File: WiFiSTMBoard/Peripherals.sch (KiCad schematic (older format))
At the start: 7 parts

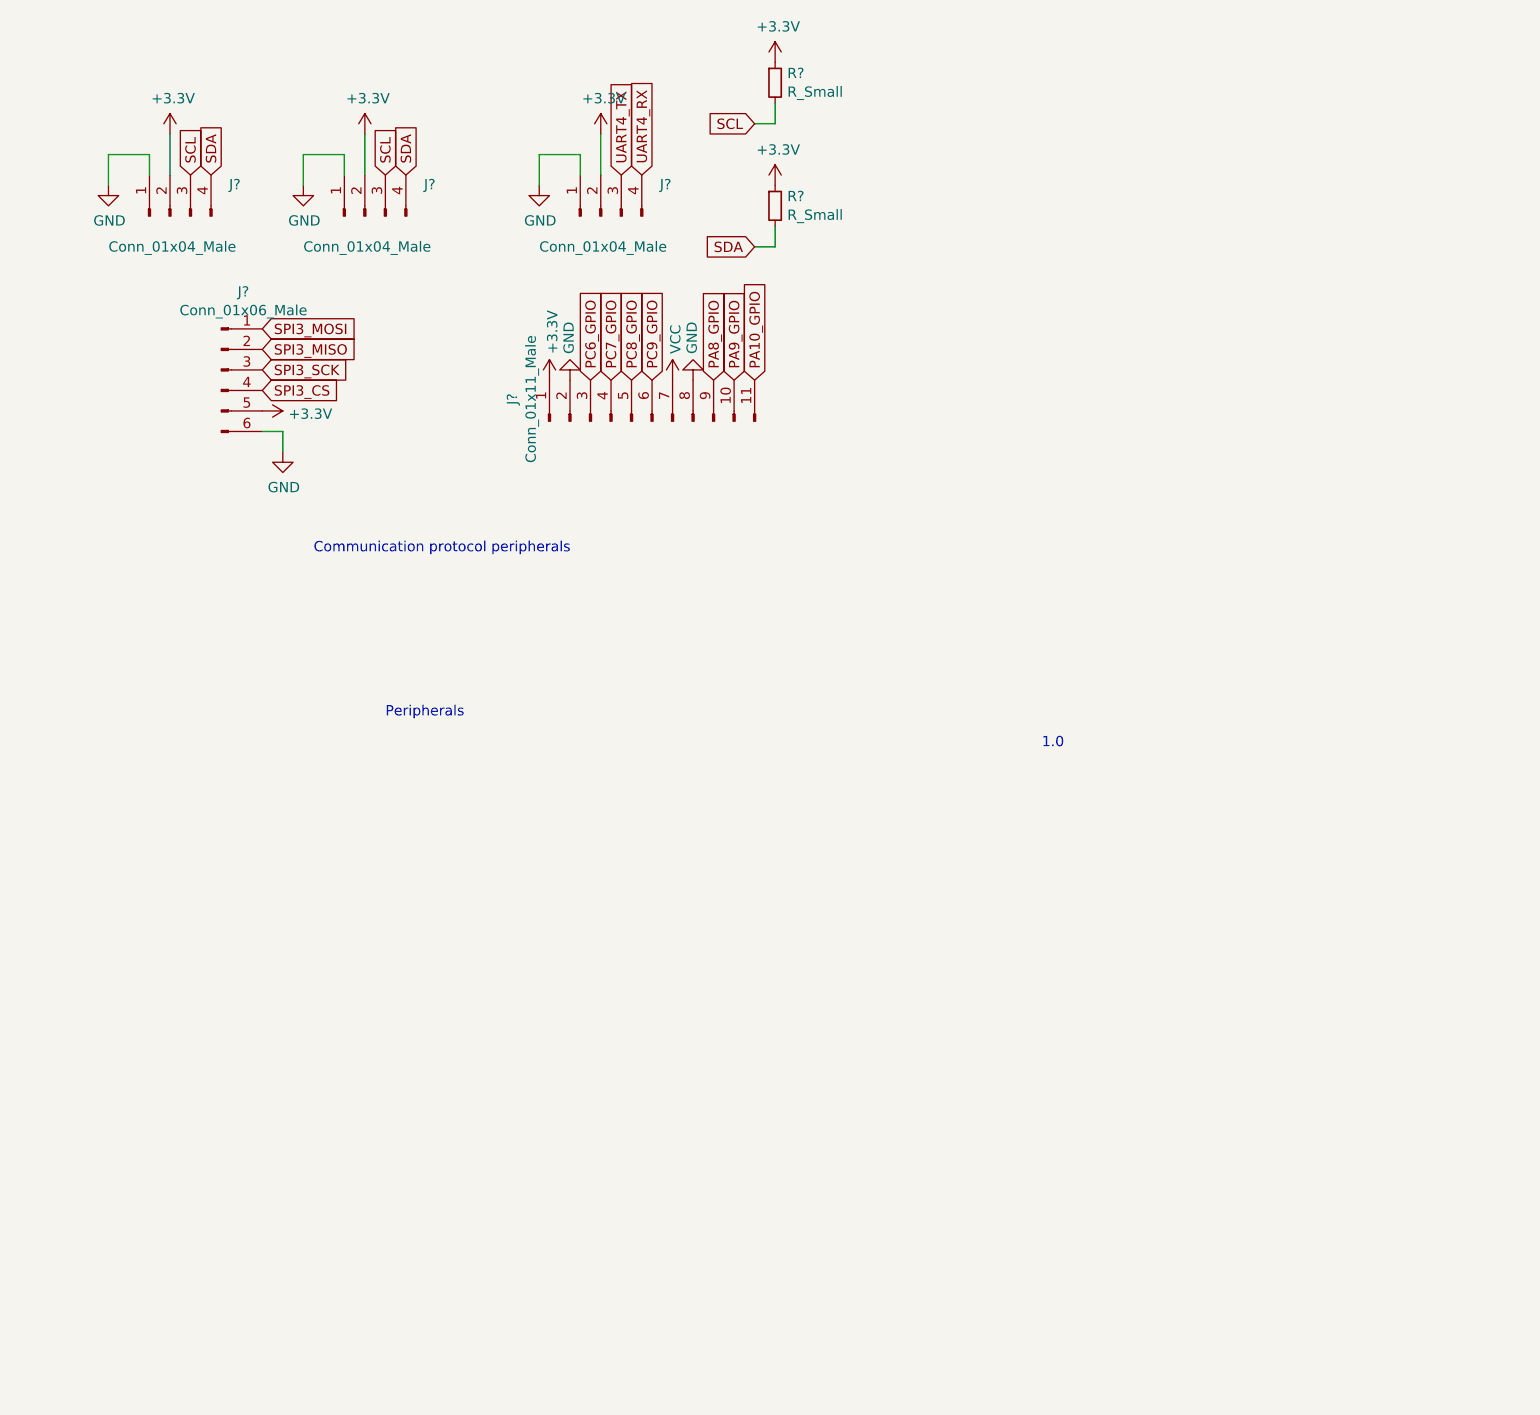
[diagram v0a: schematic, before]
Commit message: added input
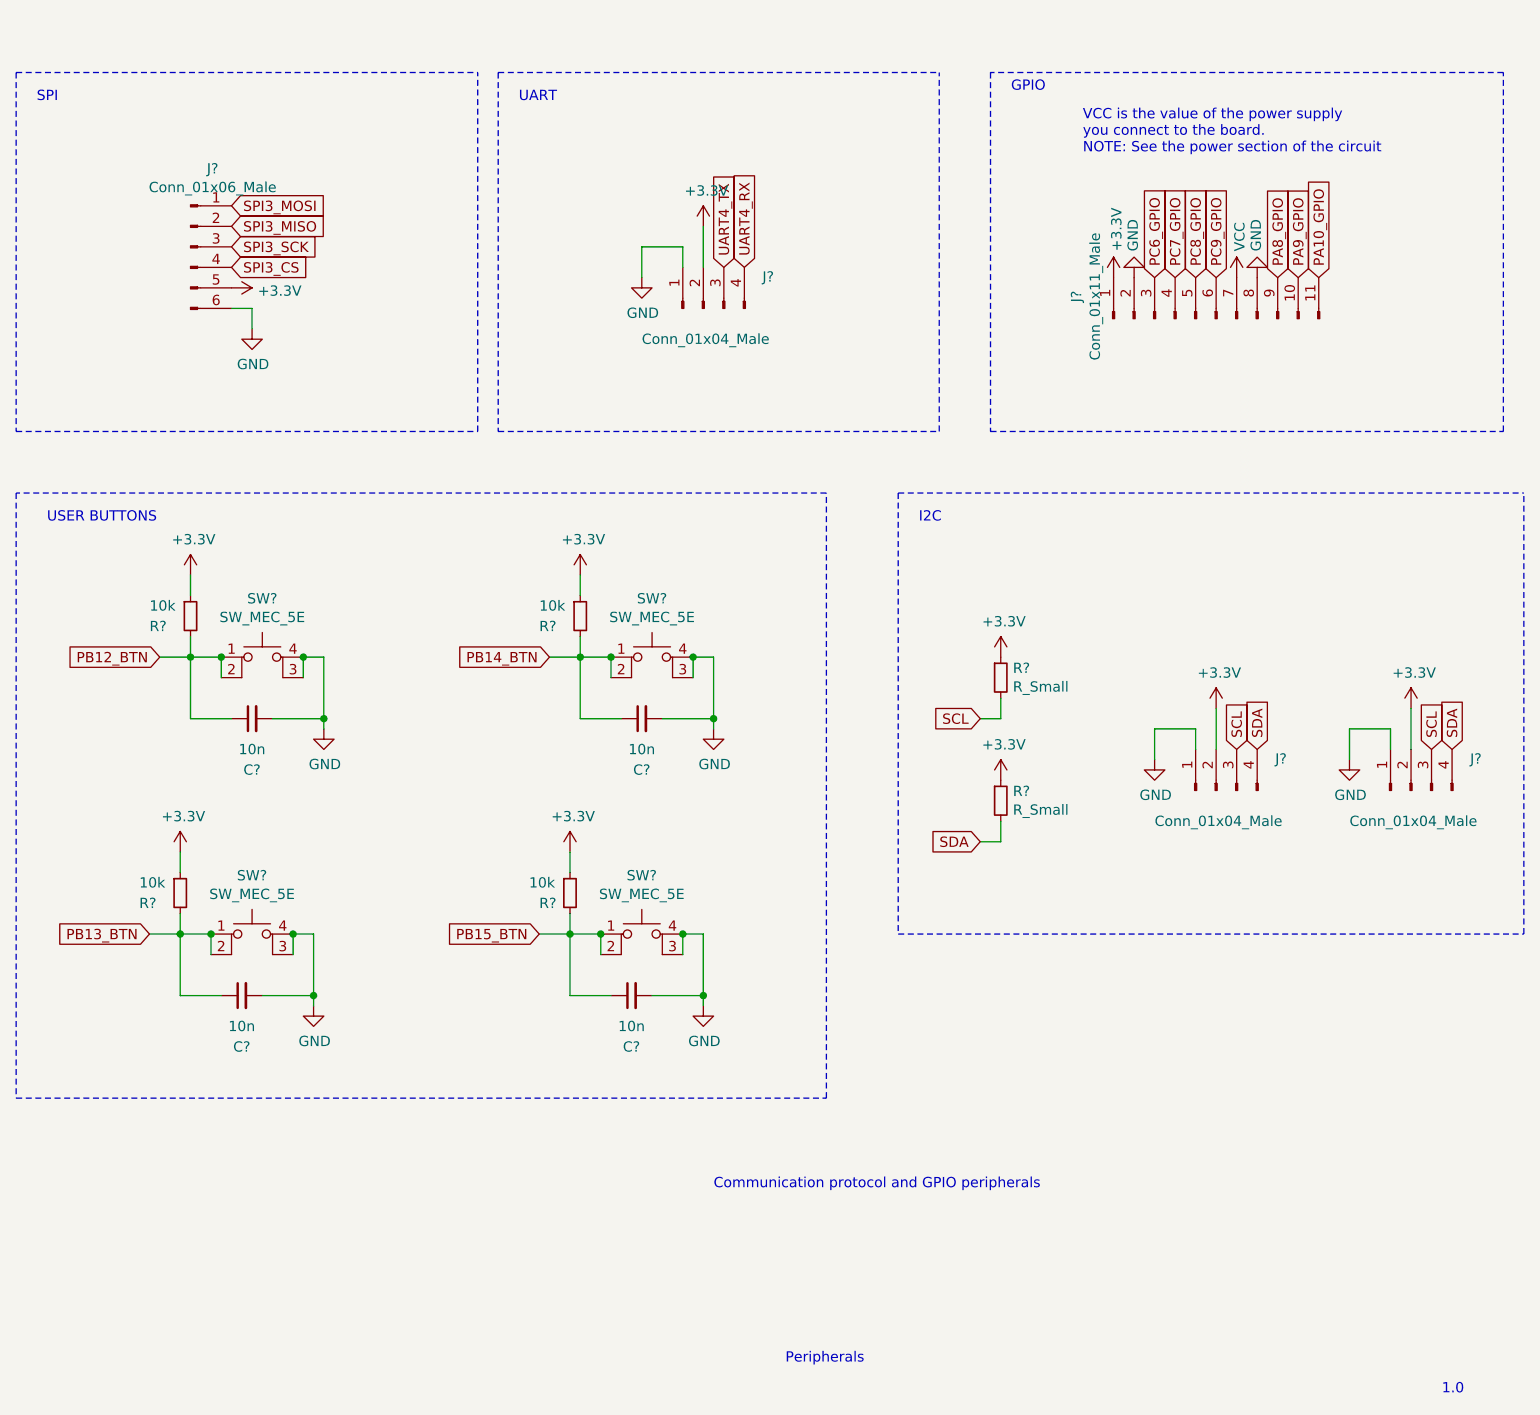
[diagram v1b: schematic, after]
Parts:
- added C? (x4): 10n, symbol Device:C_Small
- added R? (x4): 10k, symbol Device:R_Small
- added SW? (x4): SW_MEC_5E, symbol Switch:SW_MEC_5E
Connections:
- net +3V3: now also R?.1, R?.1, R?.1, R?.1
- net GND: now also C?.2, C?.2, C?.2, C?.2, SW?.3 (K), SW?.3 (K), SW?.3 (K), SW?.3 (K), SW?.4 (A), SW?.4 (A), SW?.4 (A), SW?.4 (A)
- new net PB12_BTN: C?.1, R?.2, SW?.1, SW?.2
- new net PB13_BTN: C?.1, R?.2, SW?.1, SW?.2
- new net PB14_BTN: C?.1, R?.2, SW?.1, SW?.2
- new net PB15_BTN: C?.1, R?.2, SW?.1, SW?.2
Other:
- note added: "Communication protocol and GPIO peripherals"
- note added: "GPIO"
- note added: "I2C"
- note added: "SPI"
- note added: "UART"
- note added: "USER BUTTONS"
- note added: "VCC is the value of the power supply \nyou connect to the board. \nNOTE: See the power section of the circuit"
- note removed: "Communication protocol peripherals"
- moved on the sheet: J?, R?
